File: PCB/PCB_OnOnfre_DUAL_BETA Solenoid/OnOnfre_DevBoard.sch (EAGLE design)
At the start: 29 parts, among them J1 9PIN 2.54MM, J3Y S8050, J7 8p, K1 G5Q-1-DC12, K2 G5Q-1-DC12, U2 esp12

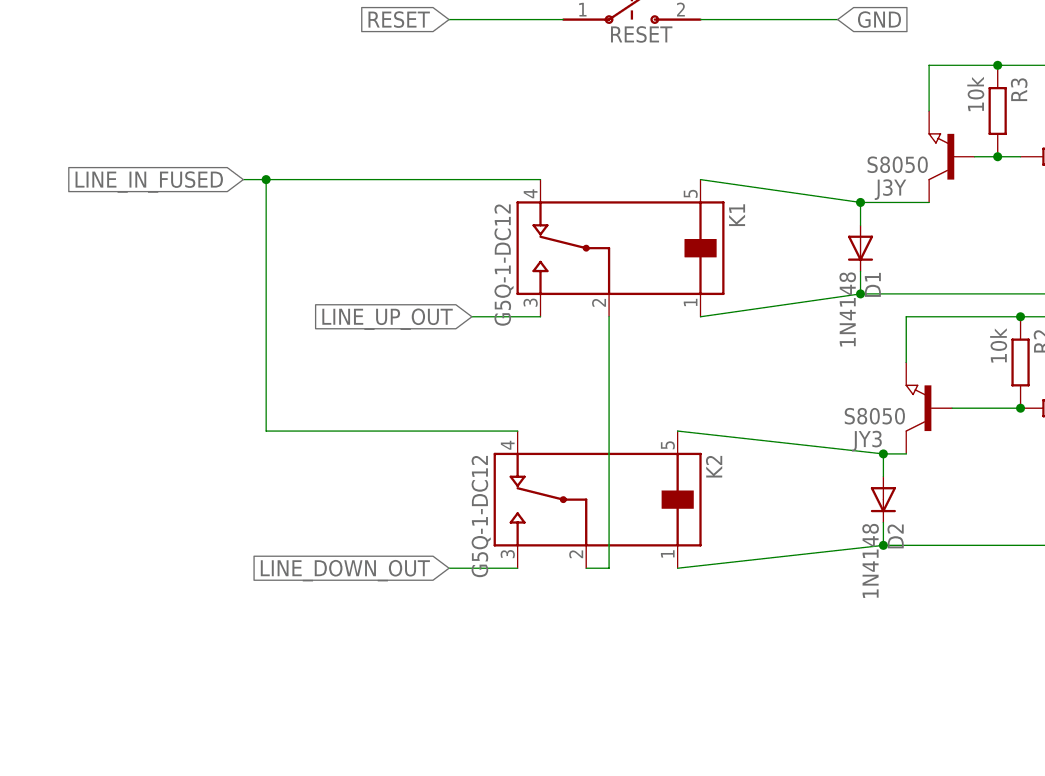
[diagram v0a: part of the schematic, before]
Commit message: s
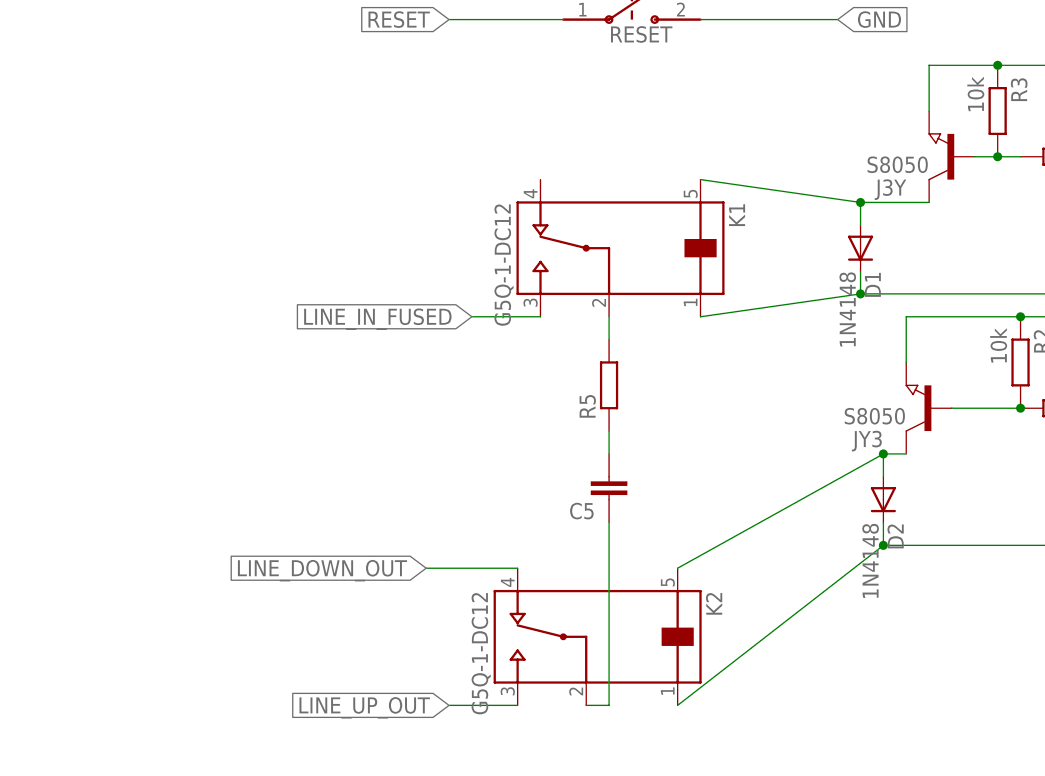
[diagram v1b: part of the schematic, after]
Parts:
- added C5: (no value), rcl:C-EU102-043X133
- added R5: (no value), resistor:R-EU_R2512
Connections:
- new net N$3: K1.2, R5.2
- new net N$4: C5.2, R5.1
- net LINE_DOWN_OUT: now also K2.4; no longer K2.3
- net LINE_IN_FUSED: now also K1.3; no longer K1.4, K2.4
- net LINE_UP_OUT: now also K2.3; no longer K1.3
- net N$2: now also C5.1; no longer K1.2
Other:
- moved on the sheet: K2
